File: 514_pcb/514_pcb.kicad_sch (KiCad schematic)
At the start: 5 parts, among them SW1 SW_SPDT

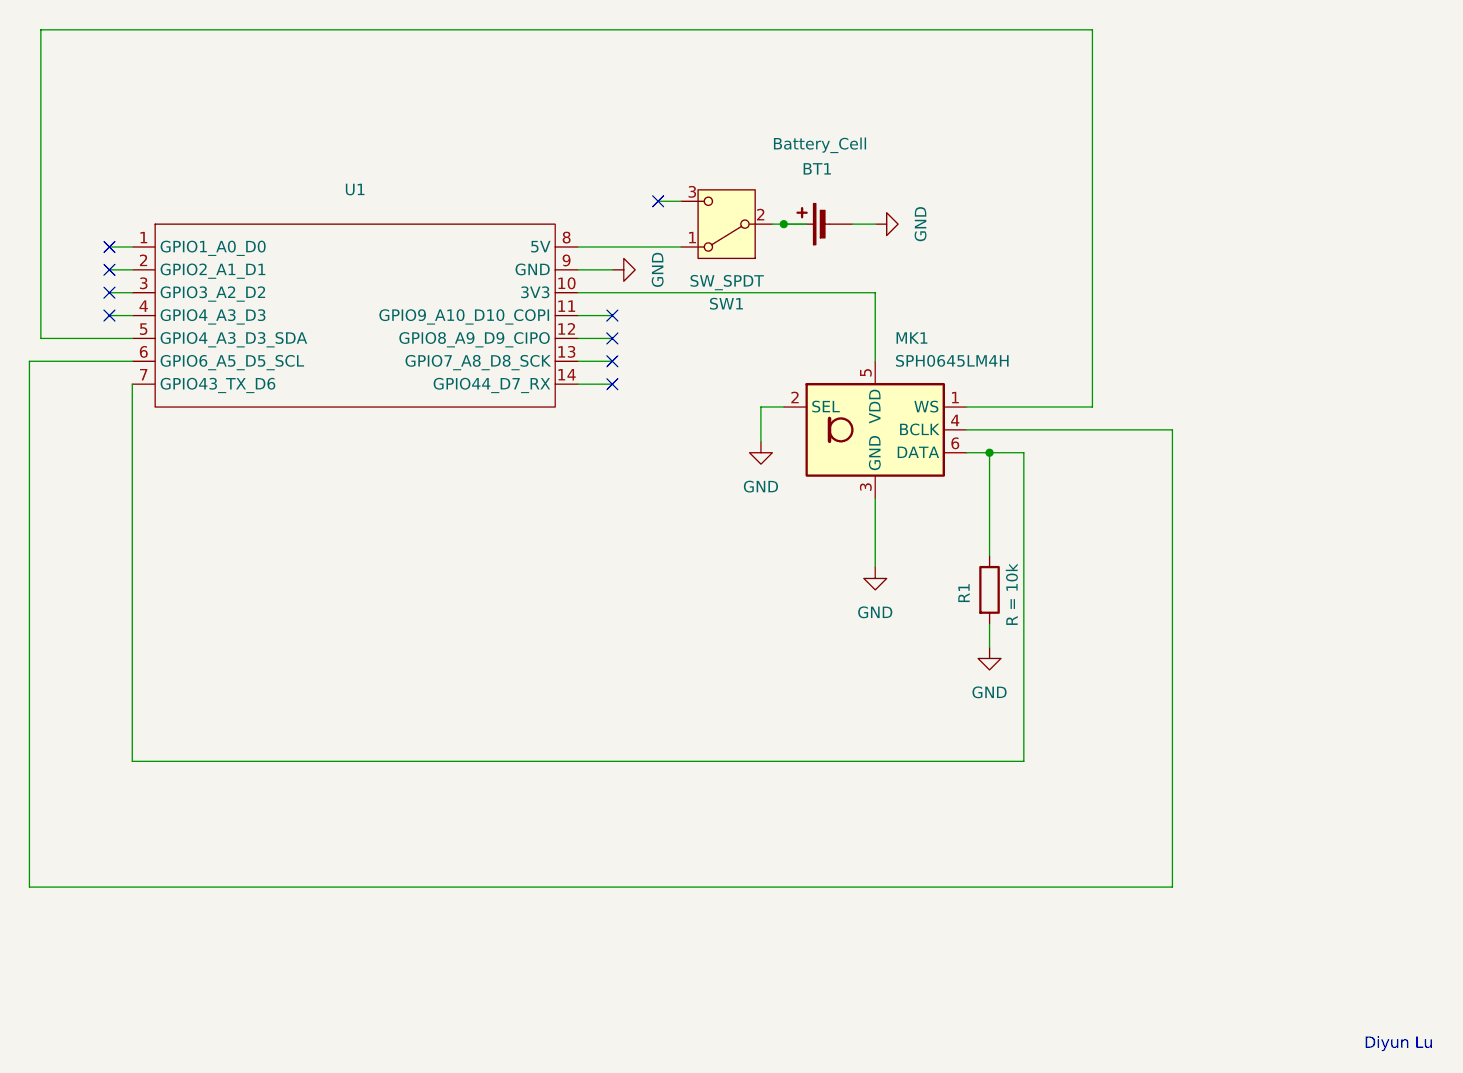
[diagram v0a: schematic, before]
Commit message: updates
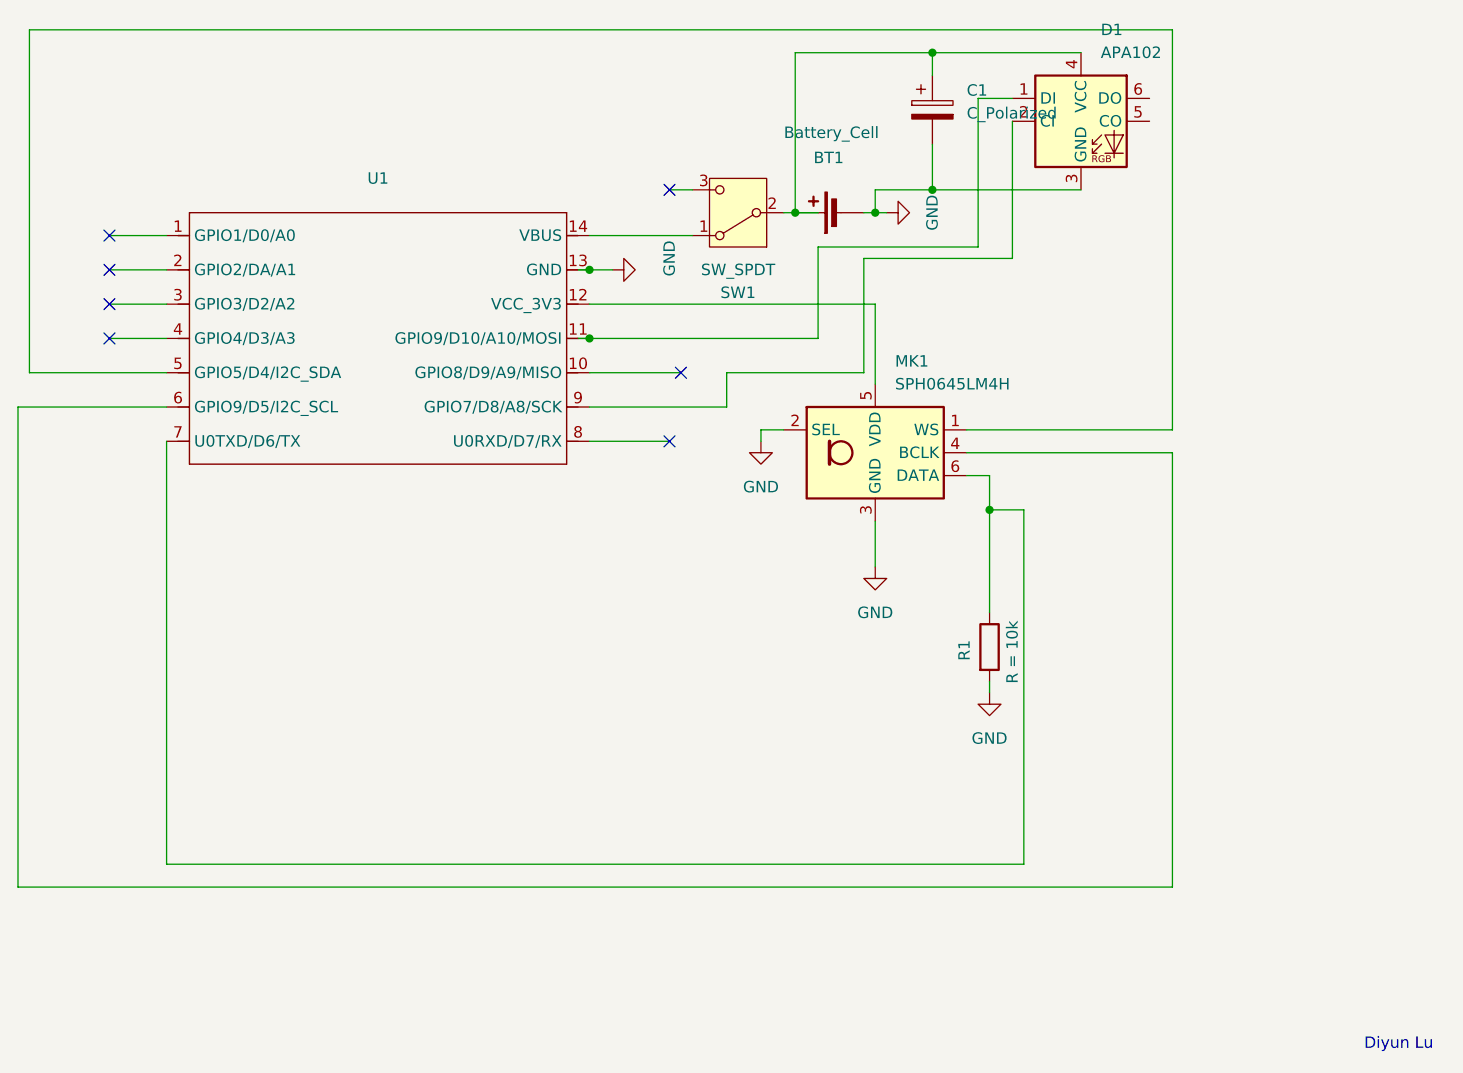
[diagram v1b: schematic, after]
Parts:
- added C1: C_Polarized, Resistor_SMD:R_0603_1608Metric_Pad0.98x0.95mm_HandSolder, symbol Device:C_Polarized
- added D1: APA102, LED_SMD:LED_RGB_5050-6, symbol LED:APA102
- U1: footprint SeeedXiao:XIAO_ESP32_SENSE -> Seeed Studio XIAO Series Library:XIAO-ESP32S3-DIP; symbol SeeedXiao:XIAO_ESP32_SENSE -> Seeed_Studio_XIAO_Series:XIAO-ESP32-S3-DIP
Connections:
- net GND: now also U1.13 (GND), C1.2, D1.3 (GND); no longer U1.9 (GND)
- net at U1.10 (GPIO8/D9/A9/MISO): no longer MK1.5 (VDD)
- net at U1.11 (GPIO9/D10/A10/MOSI): now also D1.1 (DI)
- net at U1.12 (VCC_3V3): now also MK1.5 (VDD)
- net at U1.14 (VBUS): now also SW1.1 (A)
- net at U1.8 (U0RXD/D7/RX): no longer SW1.1 (A)
- net at BT1.1 (+), SW1.2 (B): now also C1.1, D1.4 (VCC)
- new net: D1.2 (CI), U1.9 (GPIO7/D8/A8/SCK)
- no-connect marks 9 -> 7
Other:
- moved on the sheet: BT1, MK1, R1, SW1
